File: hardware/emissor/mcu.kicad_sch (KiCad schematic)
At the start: 15 parts, among them J1 I2C, SW1 RESET, SW2 BOOT, U1 ESP32-C3-MINI-1-H4X

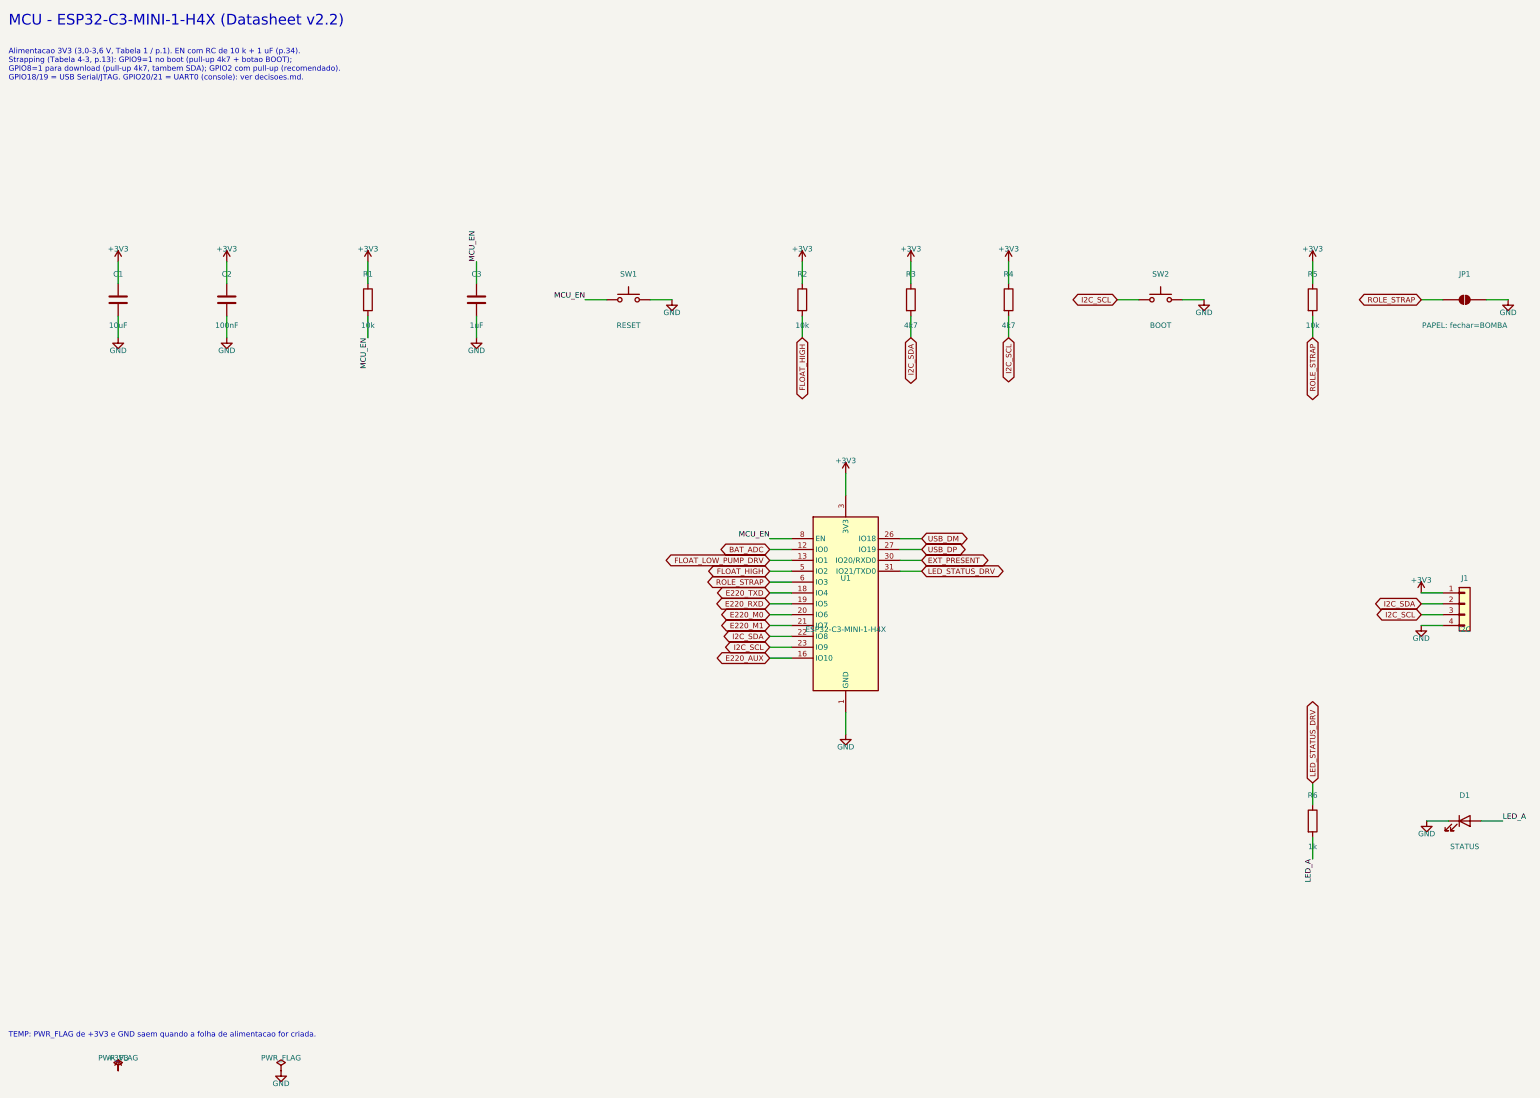
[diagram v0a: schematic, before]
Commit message: feat(hw): placas emissor e receptor com layout posicionado, 3D e STEP (hw-v0.1 em andamento)
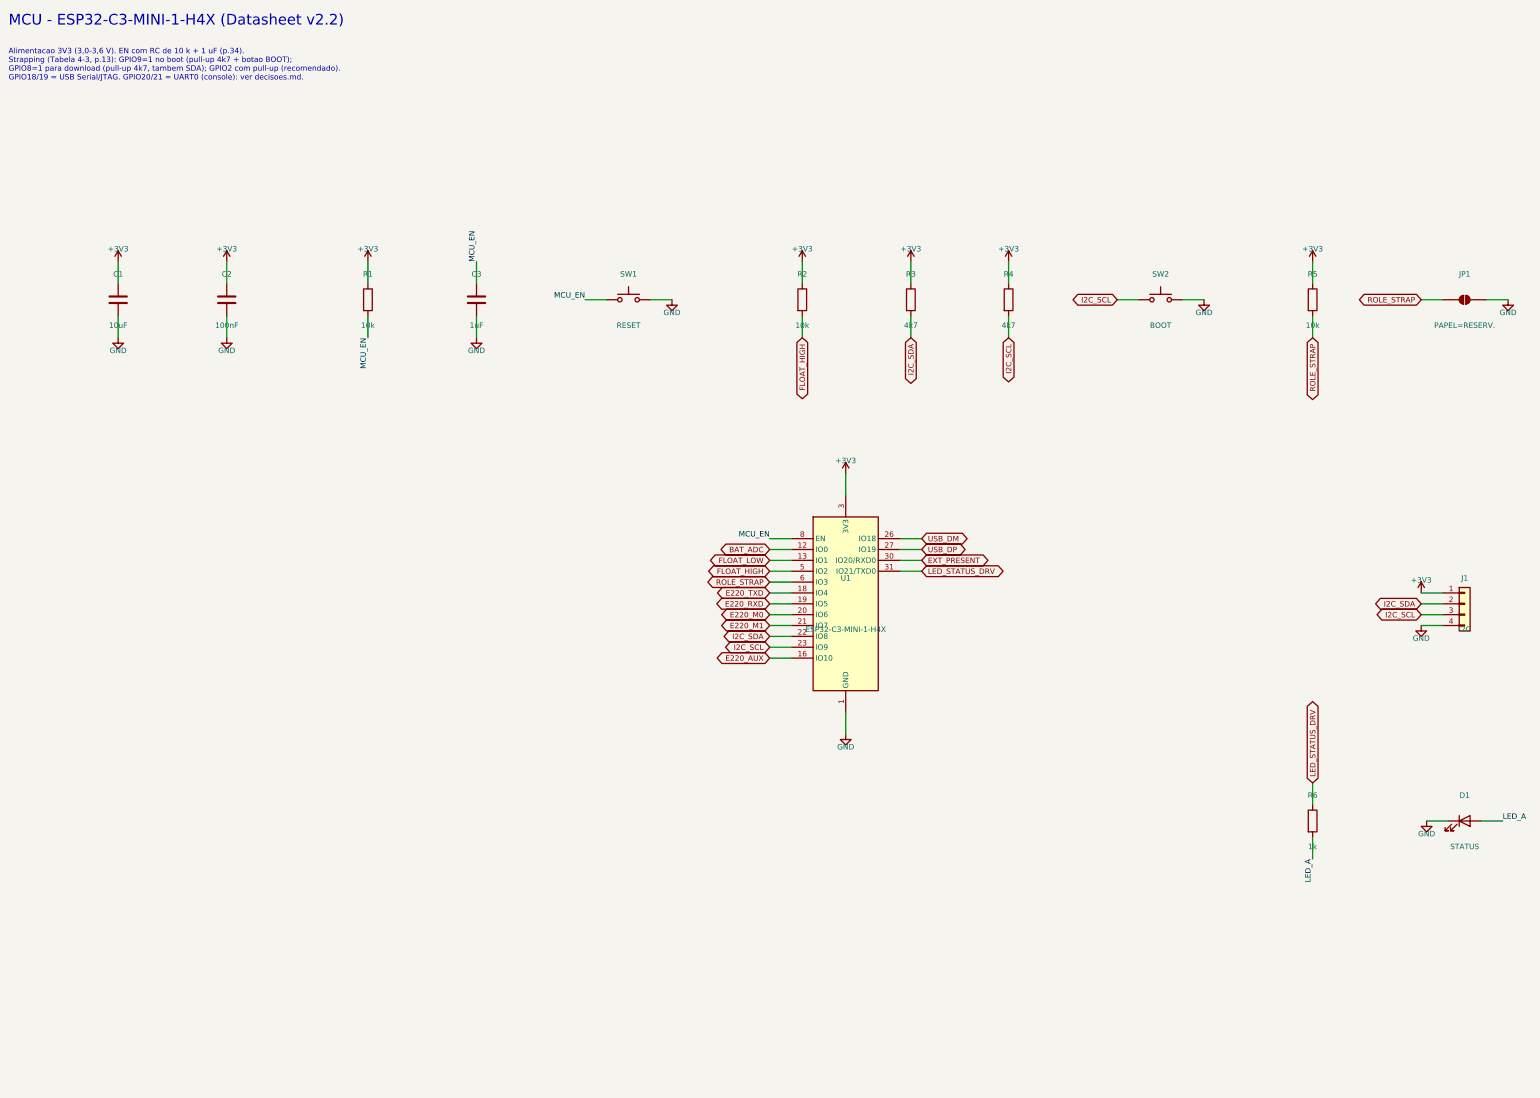
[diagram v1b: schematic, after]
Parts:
- JP1: value PAPEL: fechar=BOMBA -> PAPEL=RESERV.
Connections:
- net FLOAT_LOW_PUMP_DRV renamed FLOAT_LOW
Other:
- note added: "Alimentacao 3V3 (3,0-3,6 V). EN com RC de 10 k + 1 uF (p.34). Strapping (Tabela 4-3, p.13): GPIO9=1 no boot (pull-up 4k7 + botao BOOT); GPIO8=1 para download (pull-up 4k7, tambem SDA); GPIO2 com pull-up (recomendado). GPIO18/19 = USB Serial/JTAG. GPIO20/21 = UART0 (console): ver decisoes.md."
- note removed: "Alimentacao 3V3 (3,0-3,6 V, Tabela 1 / p.1). EN com RC de 10 k + 1 uF (p.34). Strapping (Tabela 4-3, p.13): GPIO9=1 no boot (pull-up 4k7 + botao BOOT); GPIO8=1 para download (pull-up 4k7, tambem SDA); GPIO2 com pull-up (recomendado). GPIO18/19 = USB Serial/JTAG. GPIO20/21 = UART0 (console): ver decisoes.md."
- note removed: "TEMP: PWR_FLAG de +3V3 e GND saem quando a folha de alimentacao for criada."
- title: MCU: ESP32-C3-MINI-1 -> MCU - Emissor (reservatorio)
